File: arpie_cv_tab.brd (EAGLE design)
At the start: 35.9 x 58.4 mm, 44 parts, among them IC1 MCP4726, IC2 74HC14D

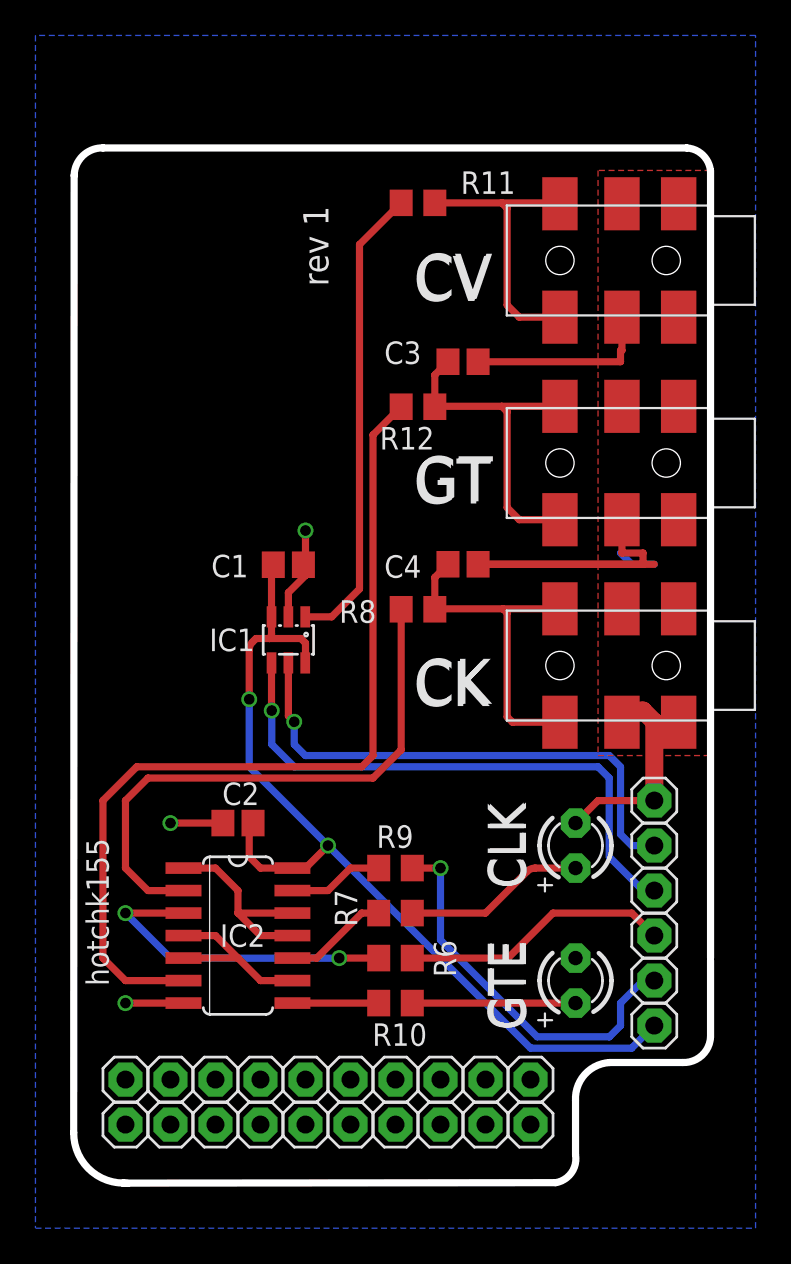
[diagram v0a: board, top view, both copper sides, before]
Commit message: v2 board
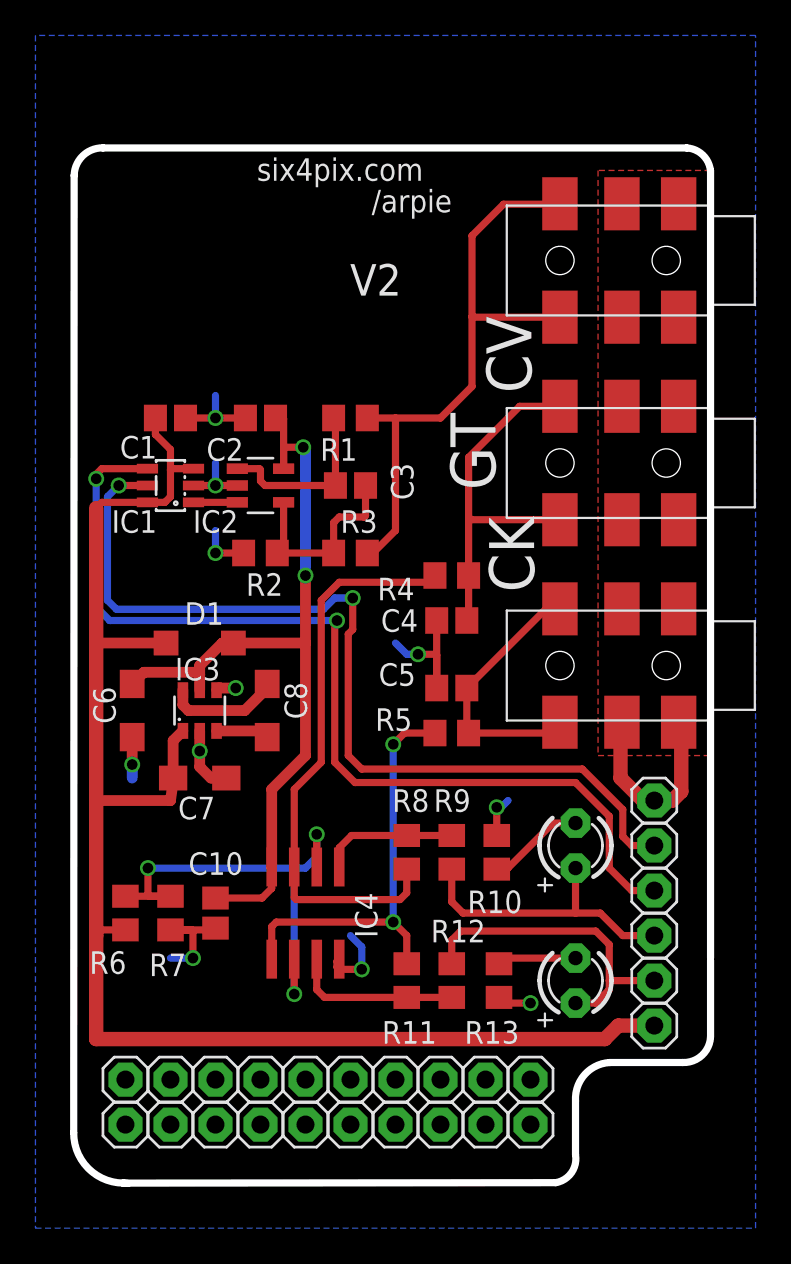
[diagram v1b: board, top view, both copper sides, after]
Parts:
- added C10, C5: (no value), resistor:C0805
- added C6: (no value), rcl:SMC_A
- added C7, C8: 10u, rcl:SMC_A
- added D1: MBR0520LT, diode:SOD123
- added IC3: LM27675M5_CHARGEPUMP, jason_eagle6:SOT23-6
- added IC4: LM358D, linear:SO08
- added R1, R2, R3, R4, R5: (no value), rcl:R0805
- added R13: 1K, rcl:R0805
- IC2: value 74HC14D -> MCP601OT; device 74xx-eu:SO14 -> linear:SOT23-5
- R11, R12, R8: value 10K -> (none)
- R6, R7, R9: value 1K -> (none)
- moved R11 43.9 mm to (79.4, 8.89), turned to 270 degrees
- moved R12 32.4 mm to (81.9, 8.89), turned to 90 degrees
- moved IC2 25.4 mm to (71.1, 36.8)
- moved C2 22.9 mm to (71.1, 40.6)
- moved R6 15.5 mm to (63.5, 12.7), turned to 270 degrees
- moved R8 13.7 mm to (79.4, 16.1), turned to 90 degrees
- moved R7 12.7 mm to (66.0, 12.7), turned to 90 degrees
- moved IC1 11.0 mm to (66.0, 36.8), turned to 90 degrees
- moved C1 10.6 mm to (66.0, 40.6), turned to 180 degrees
- moved R10 10.3 mm to (84.5, 16.1), turned to 90 degrees
- moved C3 9.44 mm to (76.2, 36.8), turned to 180 degrees
- moved CLK_LED 7.62 mm to (88.9, 8.89)
- moved GATE_LED 7.62 mm to (88.9, 16.5)
- moved R9 3.30 mm to (81.9, 16.1), turned to 270 degrees
- moved C4 3.24 mm to (81.9, 29.2), turned to 180 degrees
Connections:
- removed net N$13: IC2.13, R9.2
- removed net N$14: IC2.3, R6.2
- removed net N$6: GATE_LED.A, R10.2
- removed net N$7: IC1.1, R11.1
- removed net N$8: CLK_LED.A, R7.2
- new net +10V: C10.1, C2.2, C6.+, D1.C, IC2.5, IC3.5, IC4.8
- new net CVOUT: CVOUT.T, CVOUT.T@, R1.1, R3.1
- new net DACOUT: IC1.1, IC2.3
- new net N$11: C3.2, IC2.1, R1.2
- new net N$15: C3.1, IC2.4, R2.1, R3.2
- new net N$38: C8.+, IC3.6
- new net N$39: C8.-, IC3.3
- net +5V: now also C1.2, C7.+, D1.A, IC3.1, R6.2; no longer C1.1, C2.2, IC2.14
- net CLK_OUT: now also CLK_LED.A, R12.2; no longer R9.1
- net GATE_OUT: now also GATE_LED.A, R9.2; no longer R6.1
- net GND: now also C1.1, C10.2, C5.2, C6.-, C7.-, GND1.1, GND2.1, GND3.1, GND4.1, GND5.1, GND6.1, IC2.2, IC3.2, IC3.4, IC4.4, R10.2, R13.2, R2.2, R7.1; no longer C1.2, C3.2, CLK_LED.K, GATE_LED.K, IC2.7
- net N$1: now also IC4.2, IC4.6, R6.1, R7.2; no longer CVOUT.T, CVOUT.T@, R11.2
- net N$12: now also IC4.7, R4.1, R8.1; no longer IC2.6, R12.1
- net N$19: now also C5.1, R5.2; no longer C4.1, R8.2
- net N$2: now also CLK_LED.K, R13.1; no longer IC2.8, R10.1
- net N$20: now also C4.1, R4.2; no longer C3.1, R12.2
- net N$3: now also GATE_LED.K, R10.1; no longer IC2.10, R7.1
- net N$4: now also IC4.3, R11.2, R12.1; no longer IC2.1, IC2.11, IC2.12
- net N$5: now also IC4.5, R8.2, R9.1; no longer IC2.4, IC2.5, IC2.9
- net N$9: now also IC4.1, R11.1, R5.1; no longer IC2.2, R8.1
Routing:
- net +10V: track 0.00 -> 46.7 mm, vias 0 -> 2
- net CVOUT: track 0.00 -> 34.6 mm
- net +5V: track 52.8 -> 86.4 mm, vias 2 -> 0
- net N$7: track 26.5 -> 0.00 mm
- net SDA: track 32.2 -> 55.2 mm, vias 1 -> 2
- net SCL: track 29.6 -> 51.9 mm, vias 1 -> 2
- net N$12: track 51.1 -> 32.3 mm
- net N$14: track 18.6 -> 0.00 mm, vias 2 -> 0
- net N$15: track 0.00 -> 11.6 mm
- net N$1: track 16.2 -> 27.3 mm, vias 0 -> 3
- net N$8: track 10.2 -> 0.00 mm
- net N$11: track 0.00 -> 10.2 mm
- net N$6: track 9.21 -> 0.00 mm
- net N$9: track 32.3 -> 24.1 mm, vias 0 -> 2
- net N$38: track 0.00 -> 6.48 mm
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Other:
- board text added: "/arpie"
- board text added: "V2"
- board text added: "six4pix.com"
- board text removed: "CLK"
- board text removed: "GTE"
- board text removed: "hotchk155"
- board text removed: "rev 1"
